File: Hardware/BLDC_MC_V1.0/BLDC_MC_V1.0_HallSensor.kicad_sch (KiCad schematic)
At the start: 18 parts, among them U10 TLV9061IDBVR, U11 TLV9061IDBVR, U3 TLV9061IDBVR

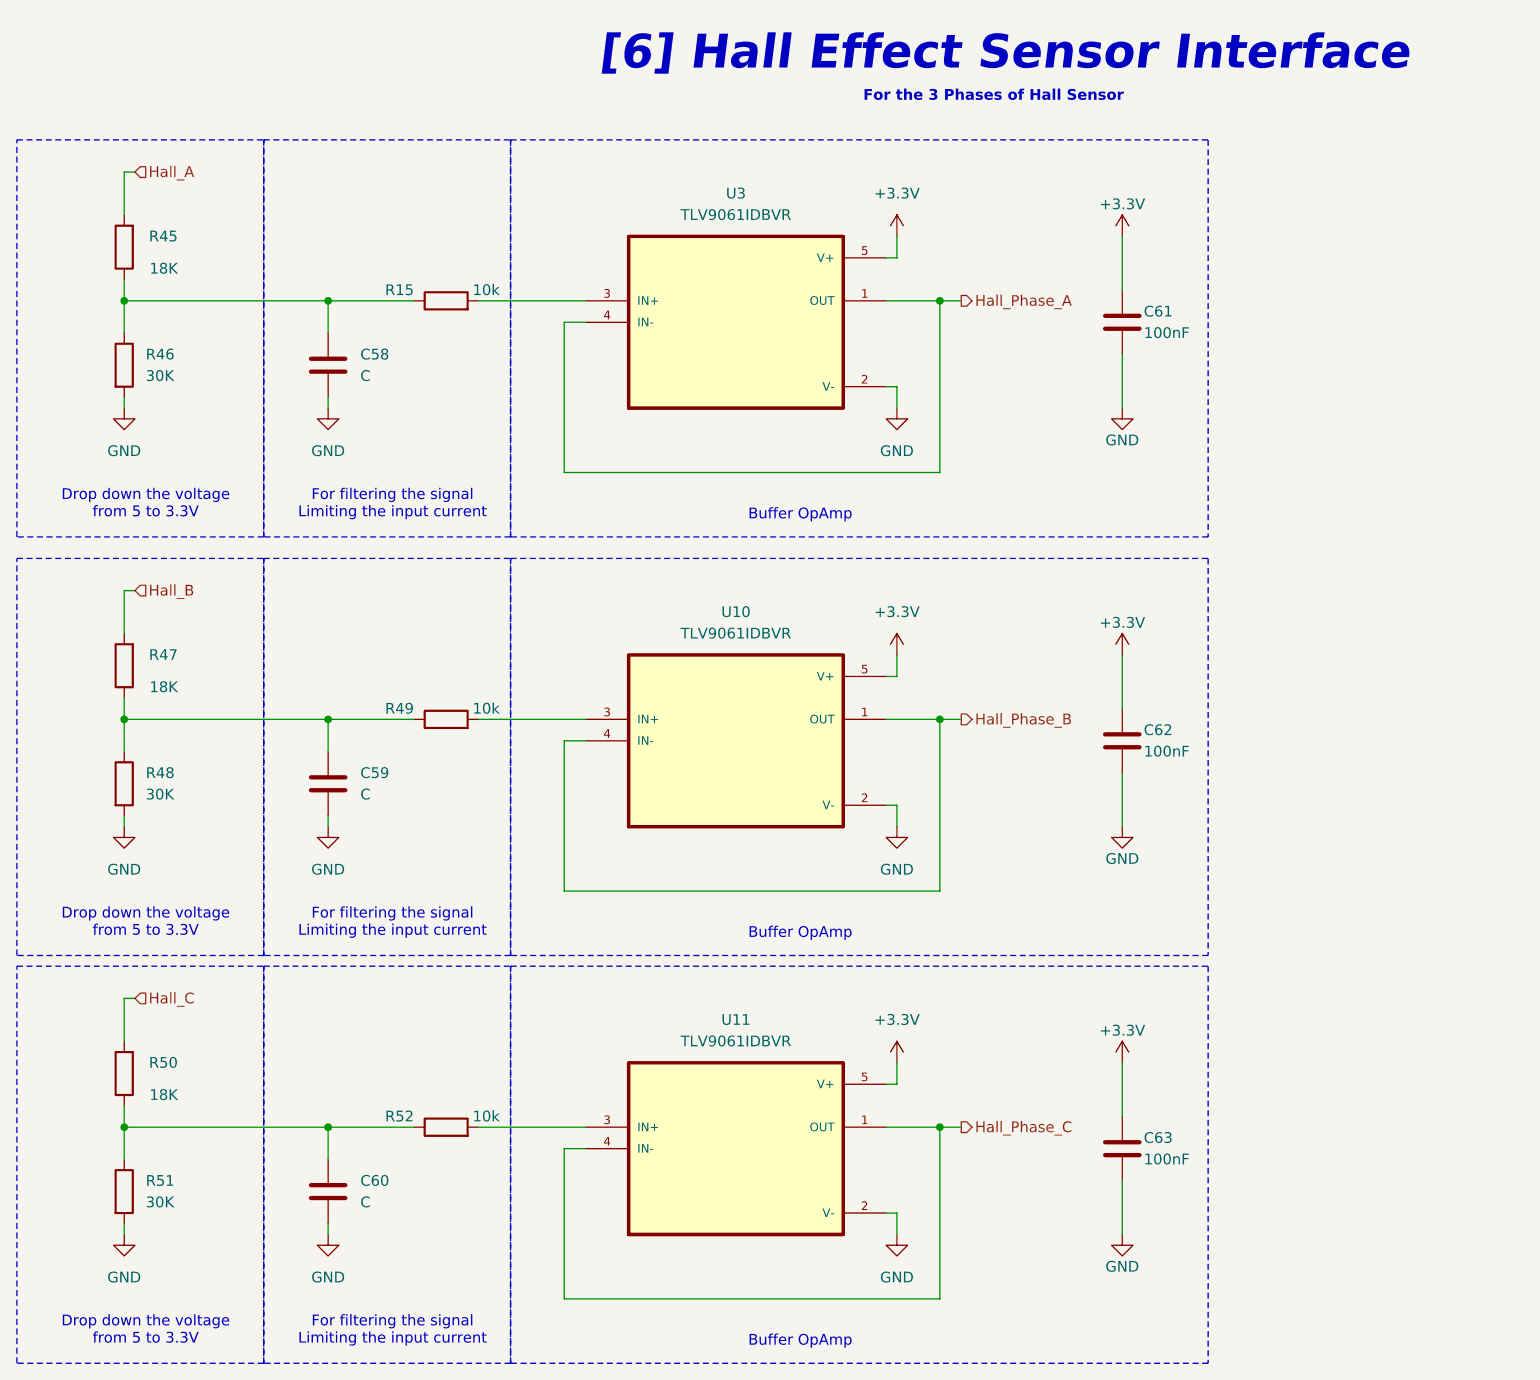
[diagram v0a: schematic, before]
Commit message: Solve all errors and wornings in project
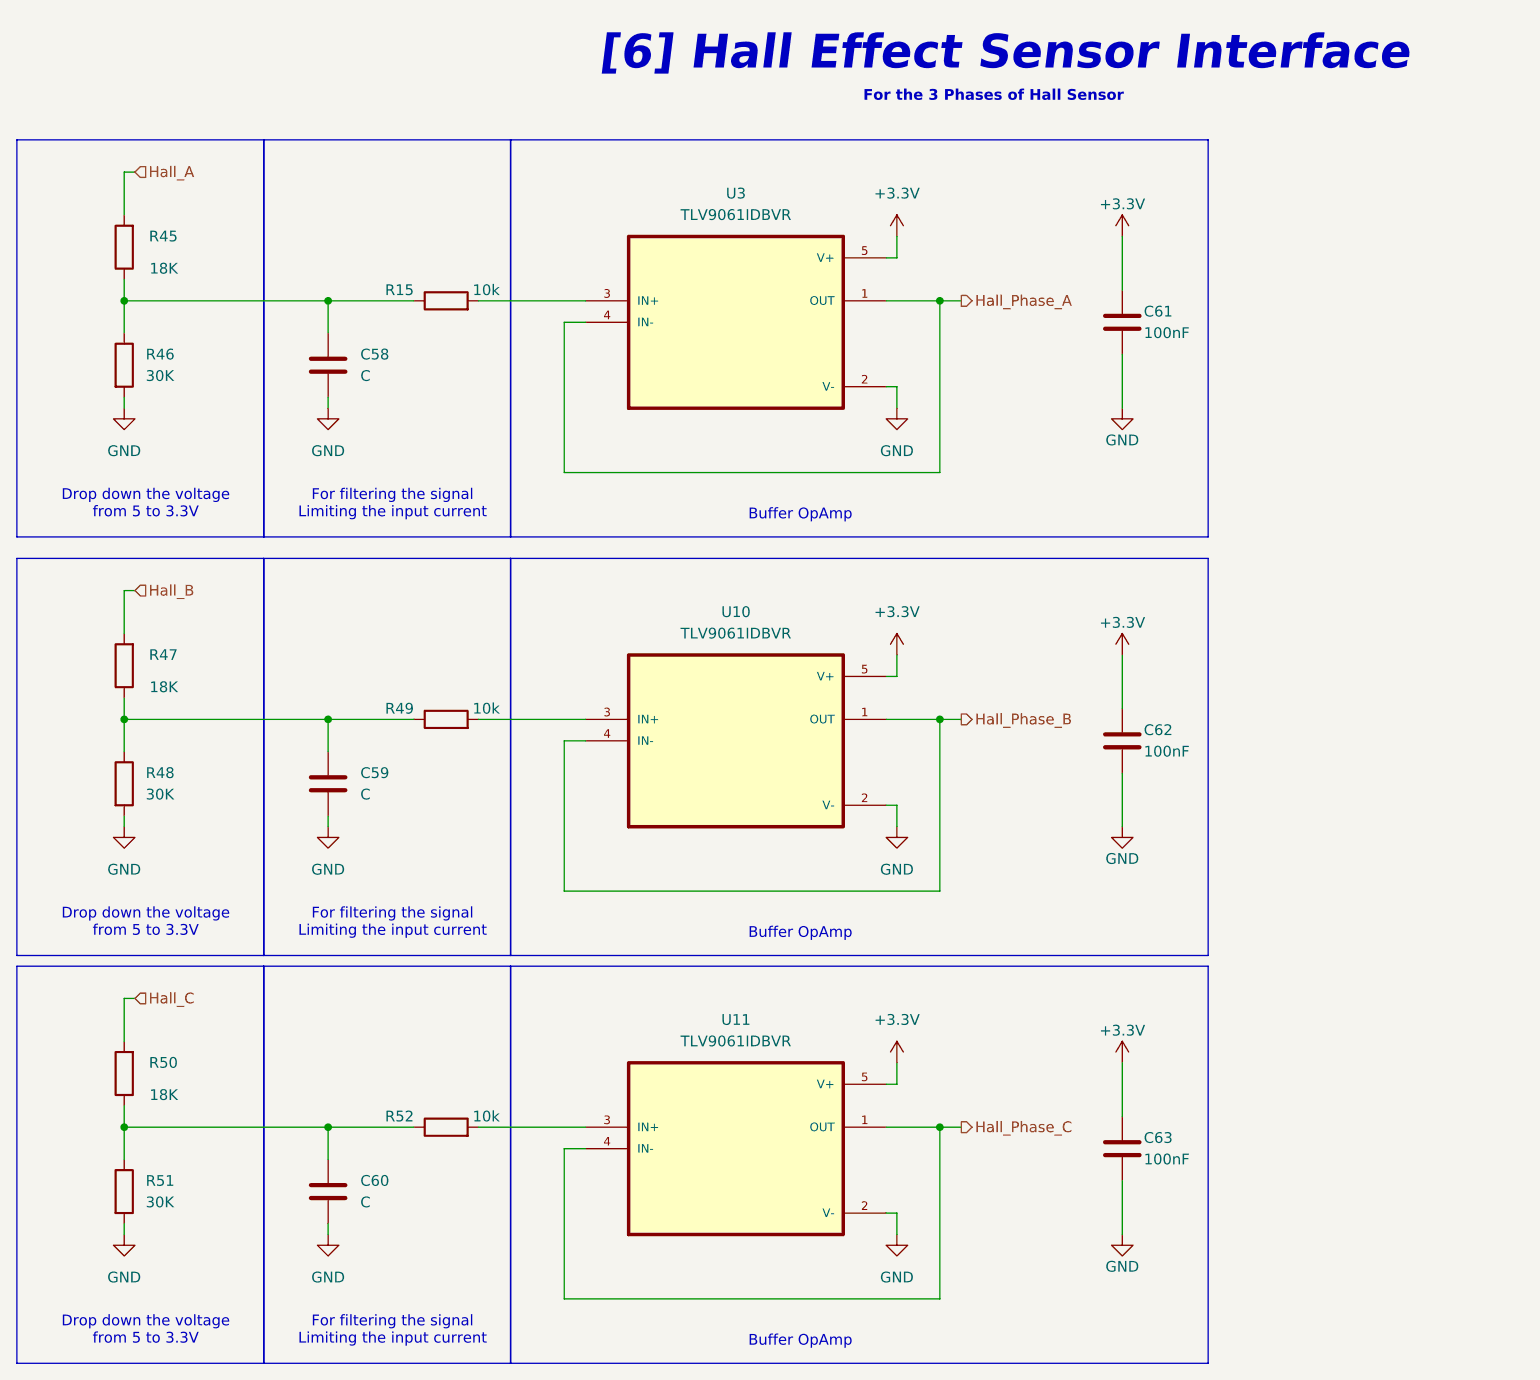
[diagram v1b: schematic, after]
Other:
- title: BLDC_MC_V1.0_HallSensor -> ${Project_Name}
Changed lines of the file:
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@@
 	(paper "A4")
 	(title_block
-		(title "BLDC_MC_V1.0_HallSensor")
+		(title "${Project_Name}")
 		(date "2026-03-05")
 		(rev "V1")
@@
 		(stroke
 			(width 0)
-			(type dash)
+			(type solid)
 		)
 		(fill
@@
 		(stroke
 			(width 0)
-			(type dash)
+			(type solid)
 		)
 		(fill
@@
 		(stroke
 			(width 0)
-			(type dash)
+			(type solid)
 		)
 		(fill
@@
 		(stroke
 			(width 0)
-			(type dash)
+			(type solid)
 		)
 		(fill
@@
 		(stroke
 			(width 0)
-			(type dash)
+			(type solid)
 		)
 		(fill
@@
 		(stroke
 			(width 0)
-			(type dash)
+			(type solid)
 		)
 		(fill
@@
 		(stroke
 			(width 0)
-			(type dash)
+			(type solid)
 		)
 		(fill
@@
 		(stroke
 			(width 0)
-			(type dash)
+			(type solid)
 		)
 		(fill
@@
 		(stroke
 			(width 0)
-			(type dash)
+			(type solid)
 		)
 		(fill
@@
 			)
 		)
-		(property "Datasheet" "https://www.lcsc.com/datasheet/C28233.pdf"
+		(property "Datasheet" "~"
 			(at 156.21 58.42 0)
 			(effects
@@
 			)
 		)
-		(property "Datasheet" "https://www.lcsc.com/datasheet/C95204.pdf"
+		(property "Datasheet" "~"
 			(at 76.2 55.88 0)
 			(effects
@@
 			)
 		)
-		(property "Datasheet" "https://www.lcsc.com/datasheet/C2906974.pdf"
+		(property "Datasheet" "~"
 			(at 38.1 49.53 0)
 			(effects
@@
 			)
 		)
-		(property "Datasheet" "https://www.lcsc.com/datasheet/C28233.pdf"
+		(property "Datasheet" "~"
 			(at 156.21 156.21 0)
 			(effects
@@
 			)
 		)
-		(property "Datasheet" "https://www.lcsc.com/datasheet/C2906974.pdf"
+		(property "Datasheet" "~"
 			(at 38.1 99.06 0)
 			(effects
@@
 			)
 		)
-		(property "Datasheet" "https://www.lcsc.com/datasheet/C95204.pdf"
+		(property "Datasheet" "~"
 			(at 76.2 153.67 0)
 			(effects
@@
 			)
 		)
-		(property "Datasheet" "https://www.lcsc.com/datasheet/C28233.pdf"
+		(property "Datasheet" "~"
 			(at 156.21 107.95 0)
 			(effects
@@
 			)
 		)
-		(property "Datasheet" "https://www.lcsc.com/datasheet/C723585.pdf"
+		(property "Datasheet" "~"
 			(at 38.1 63.5 0)
 			(effects
@@
 			)
 		)
-		(property "Datasheet" "https://www.lcsc.com/datasheet/C2906974.pdf"
+		(property "Datasheet" "~"
 			(at 38.1 147.32 0)
 			(effects
@@
 			)
 		)
-		(property "Datasheet" "https://www.lcsc.com/datasheet/C95204.pdf"
+		(property "Datasheet" "~"
 			(at 76.2 105.41 0)
 			(effects
@@
 			)
 		)
-		(property "Datasheet" "https://www.lcsc.com/datasheet/C723585.pdf"
+		(property "Datasheet" "~"
 			(at 38.1 113.03 0)
 			(effects
@@
 			)
 		)
-		(property "Datasheet" "https://www.lcsc.com/datasheet/C723585.pdf"
+		(property "Datasheet" "~"
 			(at 38.1 161.29 0)
 			(effects
